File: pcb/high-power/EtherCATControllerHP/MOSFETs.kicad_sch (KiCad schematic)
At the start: 19 parts

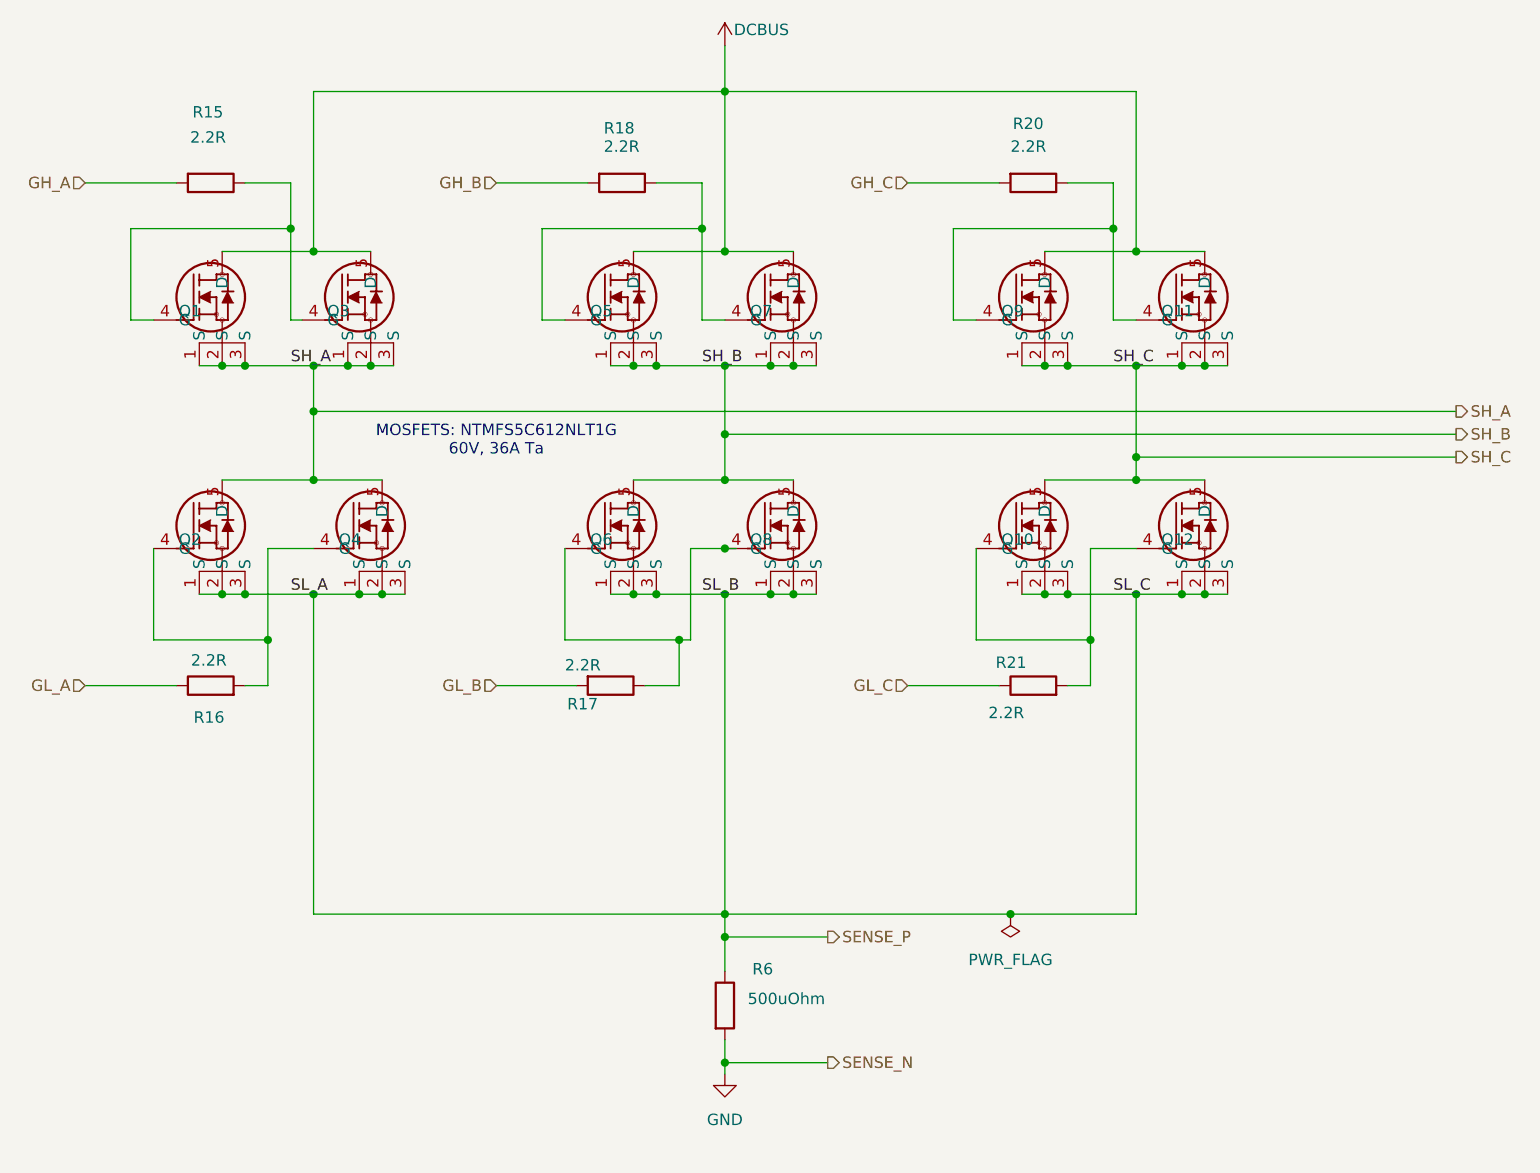
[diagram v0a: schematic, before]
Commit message: starting HP version
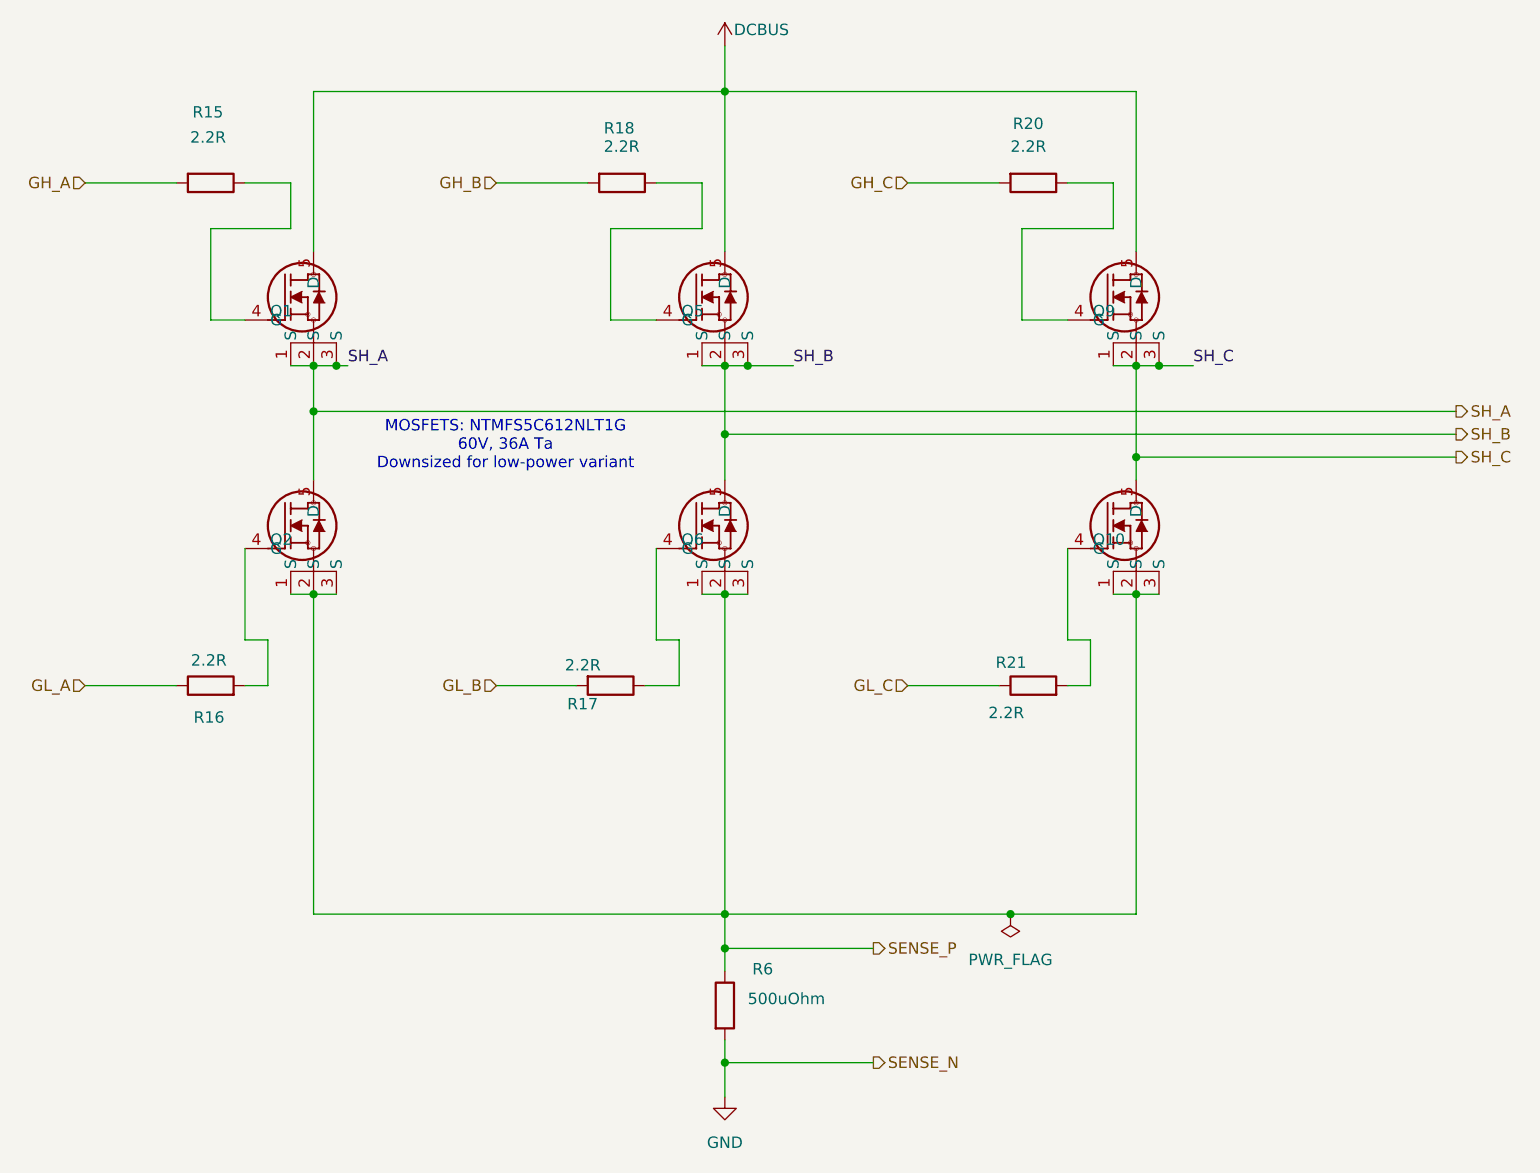
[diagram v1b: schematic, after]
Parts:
- removed Q11, Q12, Q3, Q4, Q7, Q8: ~, DFN_2NLT1G_ONS, symbol 2024-07-02_05-47-45:NTMFS5C612NLT1G
- Q1: footprint DFN_2NLT1G_ONS -> Package_SO:ONSemi_SO-8FL_488AA; LCSC Part # (none) -> C348543; LCSC Part Number C348543 -> (none)
- Q10, Q2, Q5, Q6, Q9: footprint DFN_2NLT1G_ONS -> Package_SO:ONSemi_SO-8FL_488AA
- R15, R16, R17, R18, R20, R21: LCSC Part # (none) -> C112307
- R6: LCSC Part # (none) -> C500733
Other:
- note added: "MOSFETS: NTMFS5C612NLT1G 60V, 36A Ta Downsized for low-power variant"
- note removed: "MOSFETS: NTMFS5C612NLT1G 60V, 36A Ta"
- moved on the sheet: Q1, Q10, Q2, Q5, Q6, Q9

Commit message: stash before via stitching
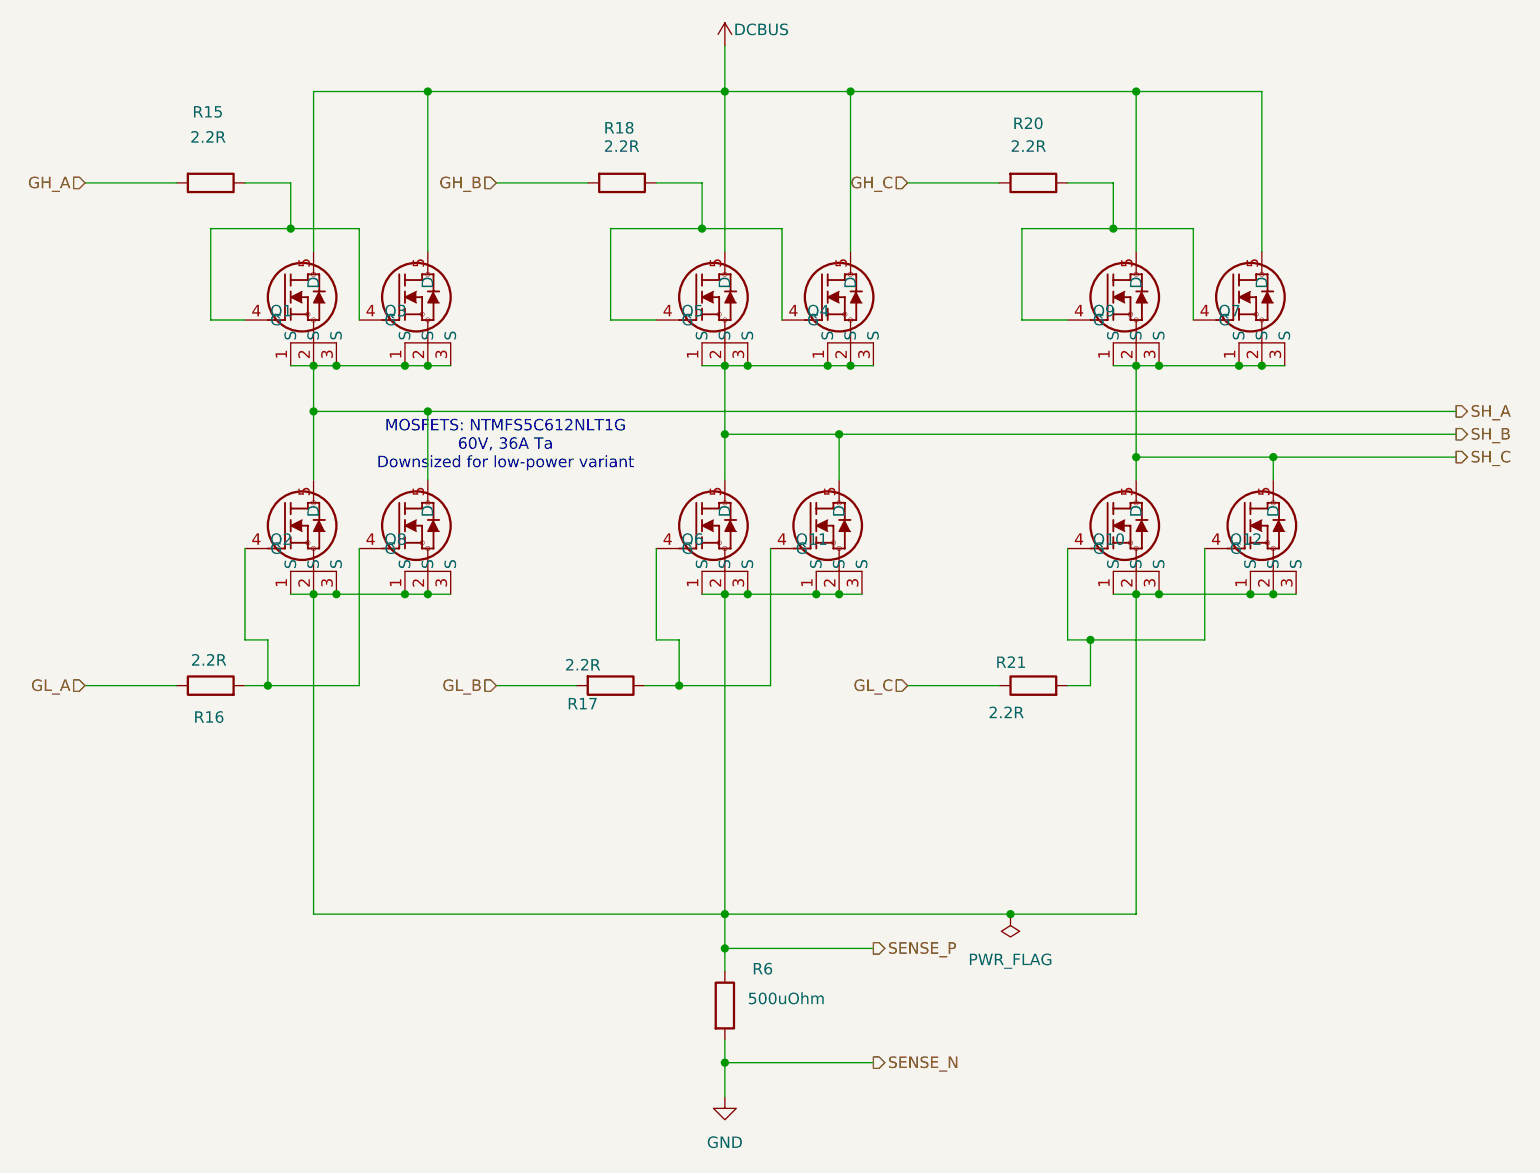
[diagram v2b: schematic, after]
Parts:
- added Q11, Q12, Q3, Q4, Q7, Q8: ~, Package_SO:ONSemi_SO-8FL_488AA, symbol 2024-07-02_05-47-45:NTMFS5C612NLT1G
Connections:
- net DCBUS: now also Q3.5 (D), Q4.5 (D), Q7.5 (D)
- net SENSE_P: now also Q11.1 (S), Q11.2 (S), Q11.3 (S), Q12.1 (S), Q12.2 (S), Q12.3 (S), Q8.1 (S), Q8.2 (S), Q8.3 (S)
- net SH_A: now also Q3.1 (S), Q3.2 (S), Q3.3 (S), Q8.5 (D)
- net SH_B: now also Q11.5 (D), Q4.1 (S), Q4.2 (S), Q4.3 (S)
- net SH_C: now also Q12.5 (D), Q7.1 (S), Q7.2 (S), Q7.3 (S)
- net at Q1.4 (G), R15.1: now also Q3.4 (G)
- net at Q10.4 (G), R21.2: now also Q12.4 (G)
- net at Q9.4 (G), R20.1: now also Q7.4 (G)
- net at Q5.4 (G), R18.1: now also Q4.4 (G)
- net at Q2.4 (G), R16.2: now also Q8.4 (G)
- net at Q6.4 (G), R17.1: now also Q11.4 (G)

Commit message: finished with HP controller
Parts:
- Q10, Q2, Q5, Q6, Q9: LCSC Part # (none) -> C348543
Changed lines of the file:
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@@
 			)
 		)
+		(property "LCSC Part #" "C348543"
+			(at 123.19 71.12 0)
+			(effects
+				(font
+					(size 1.27 1.27)
+				)
+				(hide yes)
+			)
+		)
 		(pin "1"
 		)
@@
 			)
 		)
+		(property "LCSC Part #" "C348543"
+			(at 123.19 96.52 0)
+			(effects
+				(font
+					(size 1.27 1.27)
+				)
+				(hide yes)
+			)
+		)
 		(pin "5"
 		)
@@
 			)
 		)
+		(property "LCSC Part #" "C348543"
+			(at 168.91 71.12 0)
+			(effects
+				(font
+					(size 1.27 1.27)
+				)
+				(hide yes)
+			)
+		)
 		(pin "5"
 		)
@@
 			)
 		)
+		(property "LCSC Part #" "C348543"
+			(at 168.91 96.52 0)
+			(effects
+				(font
+					(size 1.27 1.27)
+				)
+				(hide yes)
+			)
+		)
 		(pin "4"
 		)
@@
 			)
 		)
-		(property "LCSC Part #" ""
+		(property "LCSC Part #" "C348543"
 			(at 77.47 96.52 0)
 			(effects
